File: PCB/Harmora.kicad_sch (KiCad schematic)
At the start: 22 parts, among them J5 128x64 2.42 inc, U14 ATmega328p-AU, Y1 16Mhz

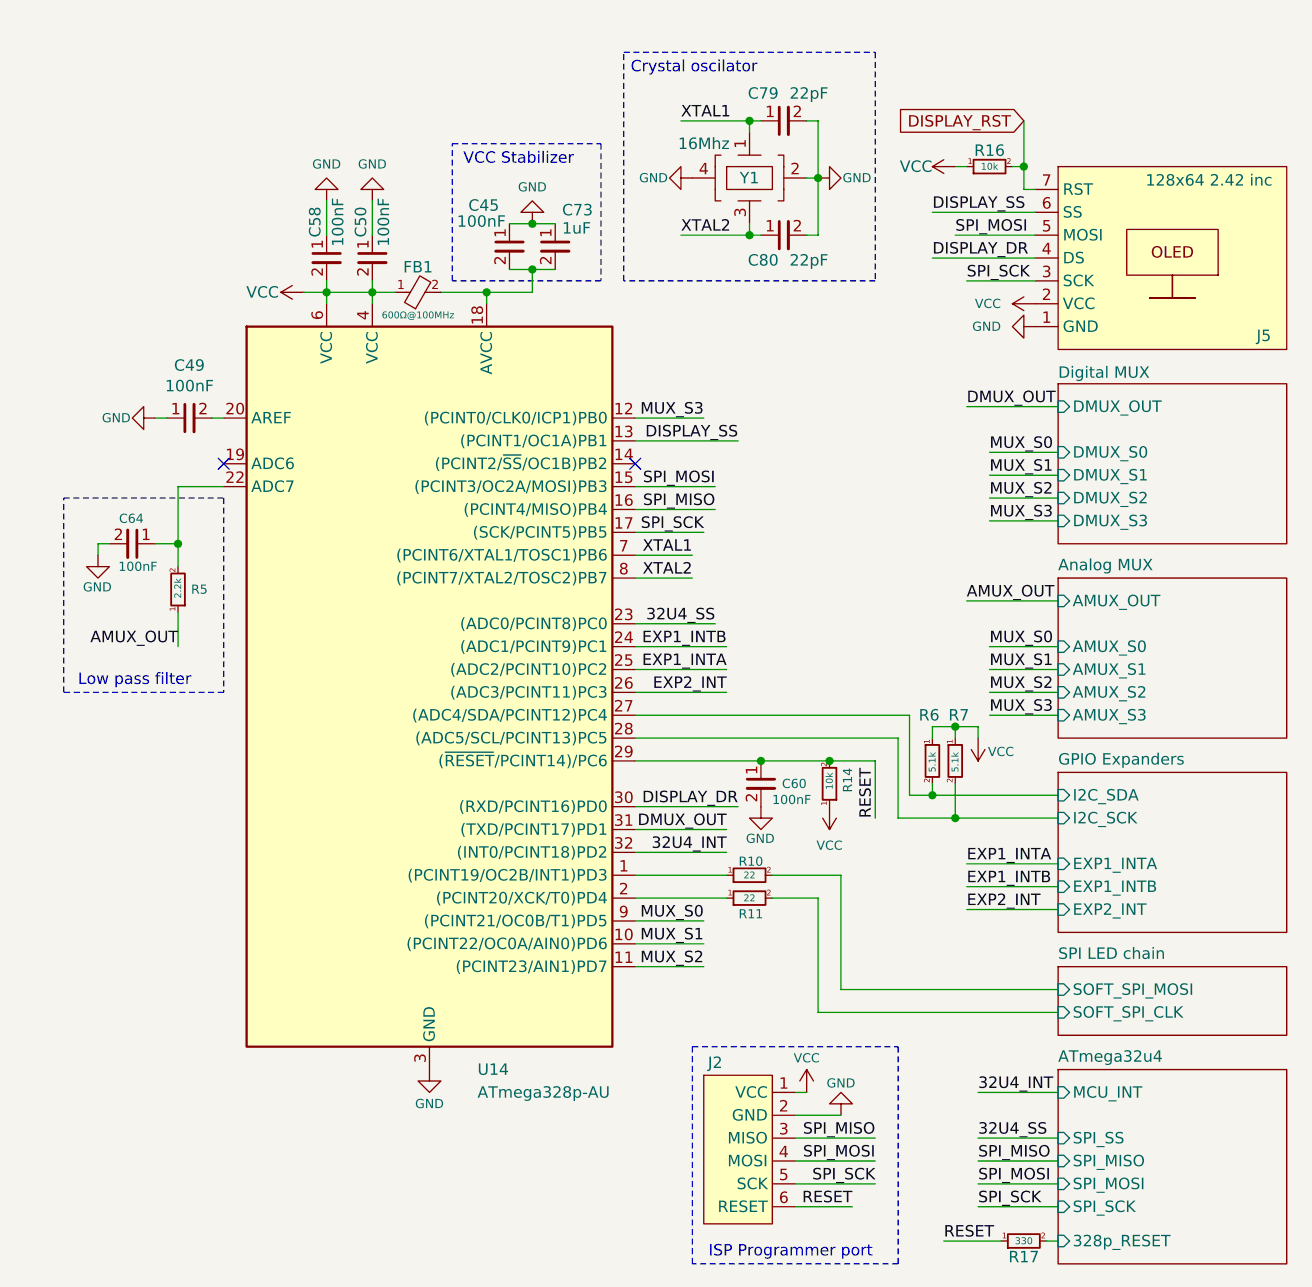
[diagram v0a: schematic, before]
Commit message: PCB V1.0 DONE
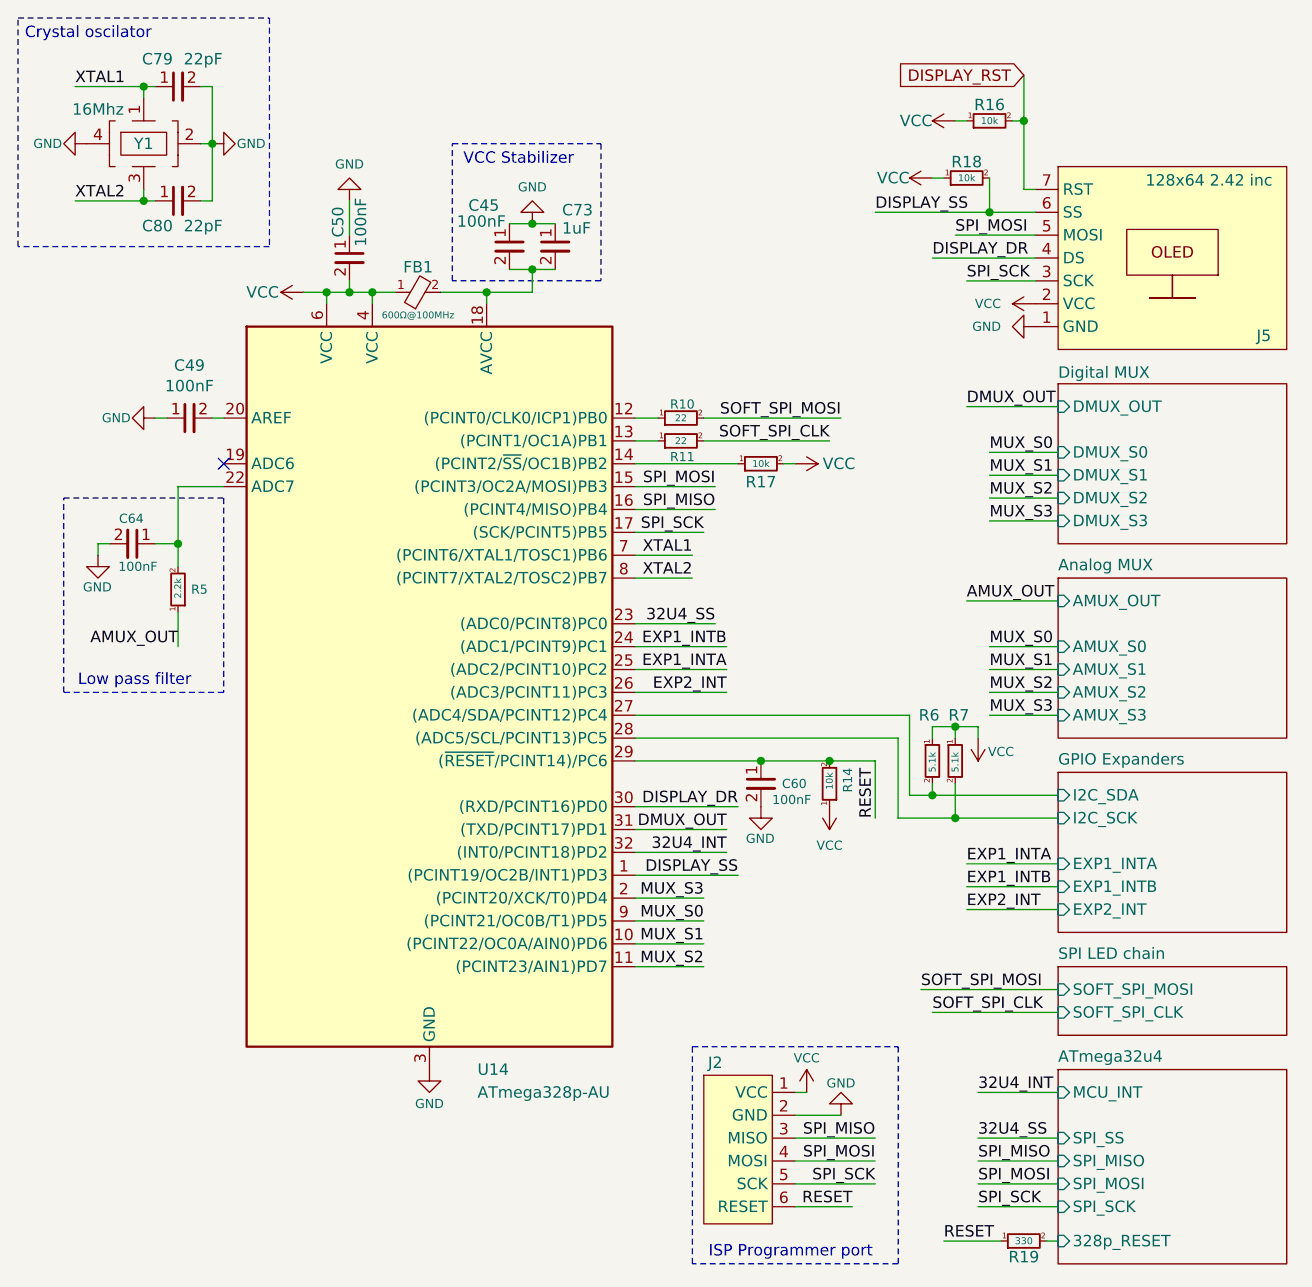
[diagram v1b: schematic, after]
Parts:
- removed C58: 100nF, Footprints:0603_C, symbol Symbols:Capacitor 0603
- added R17, R18: 10k, Footprints:0603_R, symbol Symbols:Resistor 0603
- renumbered R17 to R19
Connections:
- net DISPLAY_SS: now also U14.1 ((PCINT19/OC2B/INT1)PD3), R18.2; no longer U14.13 ((PCINT1/OC1A)PB1)
- net MUX_S3: now also U14.2 ((PCINT20/XCK/T0)PD4); no longer U14.12 ((PCINT0/CLK0/ICP1)PB0)
- net VCC: now also R17.2, R18.1
- net at R11.1: now also U14.13 ((PCINT1/OC1A)PB1); no longer U14.2 ((PCINT20/XCK/T0)PD4)
- net at R10.1: now also U14.12 ((PCINT0/CLK0/ICP1)PB0); no longer U14.1 ((PCINT19/OC2B/INT1)PD3)
- net at U14.14 ((PCINT2/~{SS}/OC1B)PB2): now also R17.1
- net SPI LED chain/SOFT_SPI_CLK renamed SOFT_SPI_CLK
- net SPI LED chain/SOFT_SPI_MOSI renamed SOFT_SPI_MOSI
- no-connect marks 2 -> 1
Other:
- moved on the sheet: C50, C79, C80, R10, R11, R16, Y1
